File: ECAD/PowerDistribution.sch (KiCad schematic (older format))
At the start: 0 parts

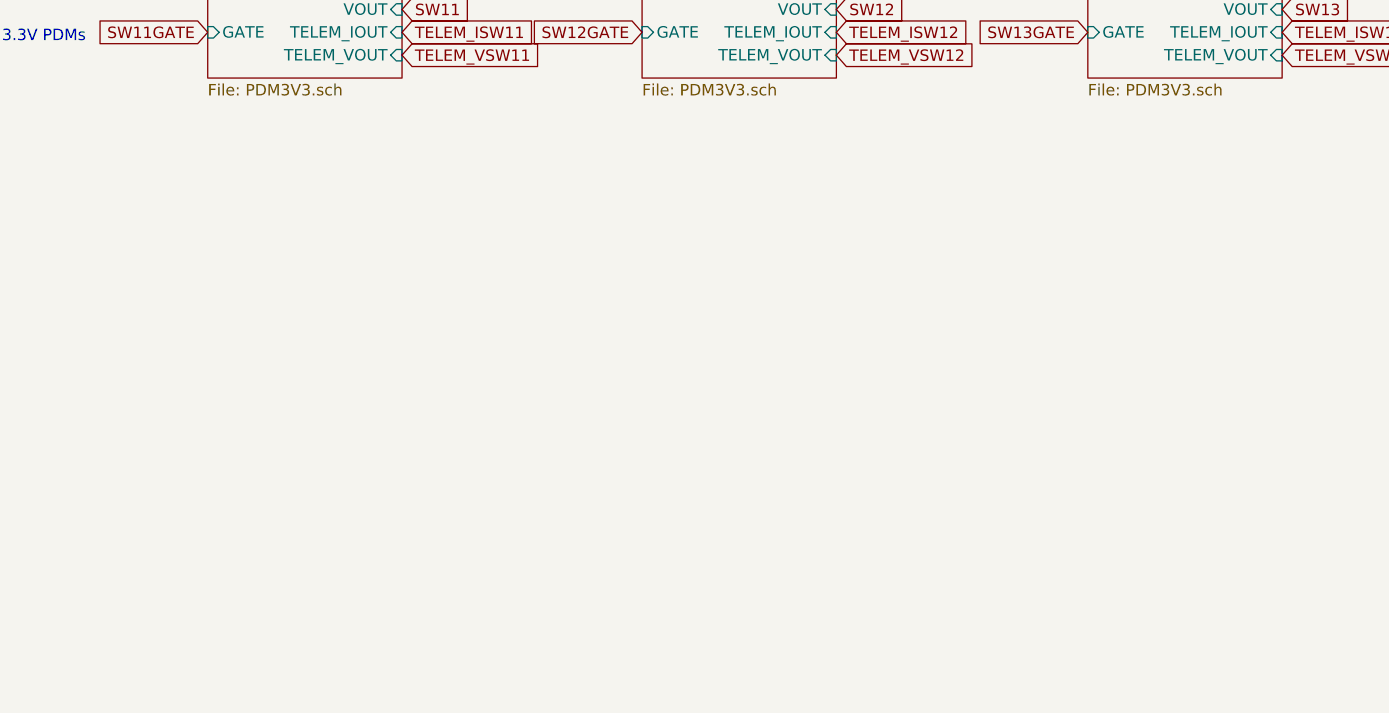
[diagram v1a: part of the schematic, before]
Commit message: add amux
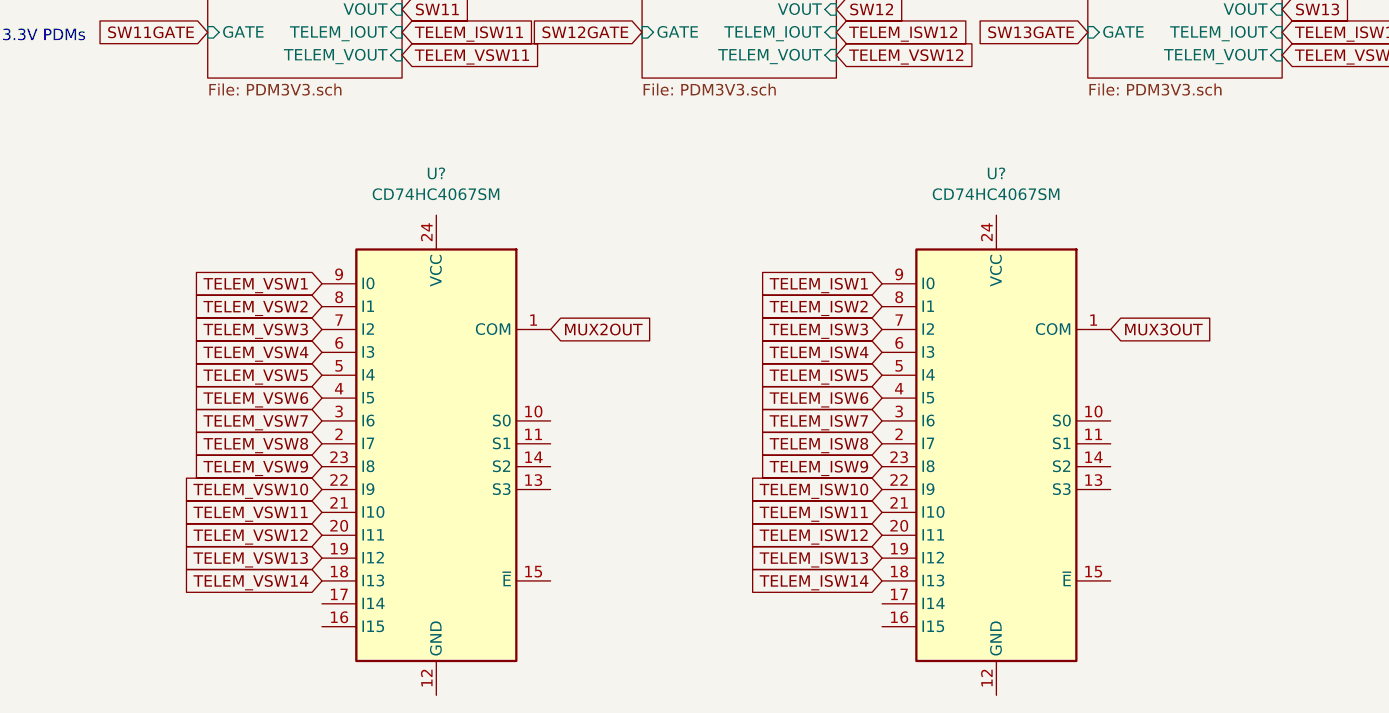
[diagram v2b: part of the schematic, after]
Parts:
- added U? (x2): CD74HC4067SM, Package_SO:SSOP-24_5.3x8.2mm_P0.65mm, symbol 74xx:CD74HC4067SM
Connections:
- net TELEM_ISW1: now also U?.9 (I0)
- net TELEM_ISW10: now also U?.22 (I9)
- net TELEM_ISW11: now also U?.21 (I10)
- net TELEM_ISW12: now also U?.20 (I11)
- net TELEM_ISW13: now also U?.19 (I12)
- net TELEM_ISW14: now also U?.18 (I13)
- net TELEM_ISW2: now also U?.8 (I1)
- net TELEM_ISW3: now also U?.7 (I2)
- net TELEM_ISW4: now also U?.6 (I3)
- net TELEM_ISW5: now also U?.5 (I4)
- net TELEM_ISW6: now also U?.4 (I5)
- net TELEM_ISW7: now also U?.3 (I6)
- net TELEM_ISW8: now also U?.2 (I7)
- net TELEM_ISW9: now also U?.23 (I8)
- net TELEM_VSW1: now also U?.9 (I0)
- net TELEM_VSW10: now also U?.22 (I9)
- net TELEM_VSW11: now also U?.21 (I10)
- net TELEM_VSW12: now also U?.20 (I11)
- net TELEM_VSW13: now also U?.19 (I12)
- net TELEM_VSW14: now also U?.18 (I13)
- net TELEM_VSW2: now also U?.8 (I1)
- net TELEM_VSW3: now also U?.7 (I2)
- net TELEM_VSW4: now also U?.6 (I3)
- net TELEM_VSW5: now also U?.5 (I4)
- net TELEM_VSW6: now also U?.4 (I5)
- net TELEM_VSW7: now also U?.3 (I6)
- net TELEM_VSW8: now also U?.2 (I7)
- net TELEM_VSW9: now also U?.23 (I8)
- new net MUX2OUT: U?.1 (COM)
- new net MUX3OUT: U?.1 (COM)
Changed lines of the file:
@@
 $Descr A4 11693 8268
 encoding utf-8
-Sheet 21 44
+Sheet 30 44
 Title "TJ Custom EPS"
 Date ""
@@
 Text Notes 1500 4400 0    50   ~ 0
 3.3V PDMs
+$Comp
+L 74xx:CD74HC4067SM U?
+U 1 1 61D9F1B4
+P 3400 6150
+AR Path="/61D9F1B4" Ref="U?"  Part="1"
+AR Path="/61E87E93/61D9F1B4" Ref="U?"  Part="1"
+F 0 "U?" H 3400 7331 50  0000 C CNN
+F 1 "CD74HC4067SM" H 3400 7240 50  0000 C CNN
+F 2 "Package_SO:SSOP-24_5.3x8.2mm_P0.65mm" H 4450 5150 50  0001 C CIN
+F 3 "http://www.ti.com/lit/ds/symlink/cd74hc4067.pdf" H 3050 7000 50  0001 C CNN
+	1    3400 6150
+	-1   0    0    -1
+$EndComp
+Text GLabel 2900 5450 0    50   Input ~ 0
+TELEM_VSW1
+Text GLabel 2900 5550 0    50   Input ~ 0
+TELEM_VSW2
+Text GLabel 2900 5650 0    50   Input ~ 0
+TELEM_VSW3
+Text GLabel 2900 5750 0    50   Input ~ 0
+TELEM_VSW4
+Text GLabel 2900 5850 0    50   Input ~ 0
+TELEM_VSW5
+Text GLabel 2900 5950 0    50   Input ~ 0
+TELEM_VSW6
+Text GLabel 2900 6050 0    50   Input ~ 0
+TELEM_VSW7
+Text GLabel 2900 6150 0    50   Input ~ 0
+TELEM_VSW8
+Text GLabel 2900 6250 0    50   Input ~ 0
+TELEM_VSW9
+Text GLabel 2900 6350 0    50   Input ~ 0
+TELEM_VSW10
+Text GLabel 2900 6450 0    50   Input ~ 0
+TELEM_VSW11
+Text GLabel 2900 6550 0    50   Input ~ 0
+TELEM_VSW12
+Text GLabel 2900 6650 0    50   Input ~ 0
+TELEM_VSW13
+Text GLabel 2900 6750 0    50   Input ~ 0
+TELEM_VSW14
+$Comp
+L 74xx:CD74HC4067SM U?
+U 1 1 61DC574F
+P 5850 6150
+AR Path="/61DC574F" Ref="U?"  Part="1"
+AR Path="/61E87E93/61DC574F" Ref="U?"  Part="1"
+F 0 "U?" H 5850 7331 50  0000 C CNN
+F 1 "CD74HC4067SM" H 5850 7240 50  0000 C CNN
+F 2 "Package_SO:SSOP-24_5.3x8.2mm_P0.65mm" H 6900 5150 50  0001 C CIN
+F 3 "http://www.ti.com/lit/ds/symlink/cd74hc4067.pdf" H 5500 7000 50  0001 C CNN
+	1    5850 6150
+	-1   0    0    -1
+$EndComp
+Text GLabel 5350 5450 0    50   Input ~ 0
+TELEM_ISW1
+Text GLabel 5350 5550 0    50   Input ~ 0
+TELEM_ISW2
+Text GLabel 5350 5650 0    50   Input ~ 0
+TELEM_ISW3
+Text GLabel 5350 5750 0    50   Input ~ 0
+TELEM_ISW4
+Text GLabel 5350 5850 0    50   Input ~ 0
+TELEM_ISW5
+Text GLabel 5350 5950 0    50   Input ~ 0
+TELEM_ISW6
+Text GLabel 5350 6050 0    50   Input ~ 0
+TELEM_ISW7
+Text GLabel 5350 6150 0    50   Input ~ 0
+TELEM_ISW8
+Text GLabel 5350 6250 0    50   Input ~ 0
+TELEM_ISW9
+Text GLabel 5350 6350 0    50   Input ~ 0
+TELEM_ISW10
+Text GLabel 5350 6450 0    50   Input ~ 0
+TELEM_ISW11
+Text GLabel 5350 6550 0    50   Input ~ 0
+TELEM_ISW12
+Text GLabel 5350 6650 0    50   Input ~ 0
+TELEM_ISW13
+Text GLabel 5350 6750 0    50   Input ~ 0
+TELEM_ISW14
+Text GLabel 3900 5650 2    50   Input ~ 0
+MUX2OUT
+Text GLabel 6350 5650 2    50   Input ~ 0
+MUX3OUT
 $EndSCHEMATC
